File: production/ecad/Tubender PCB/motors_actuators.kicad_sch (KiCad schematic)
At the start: 5 parts, among them J2 1729157, J3 1729157, J4 1729157, J5 1729157, J6 1729186

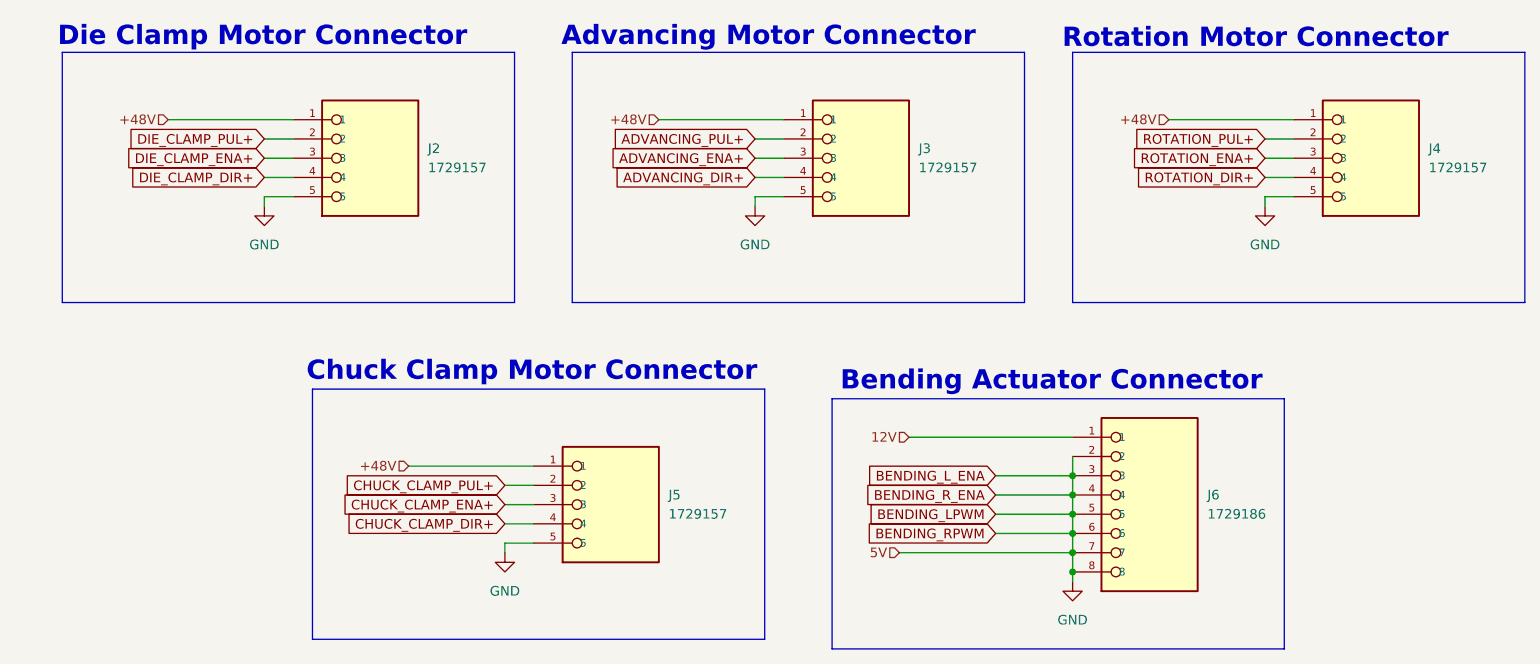
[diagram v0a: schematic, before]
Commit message: final for rev 1
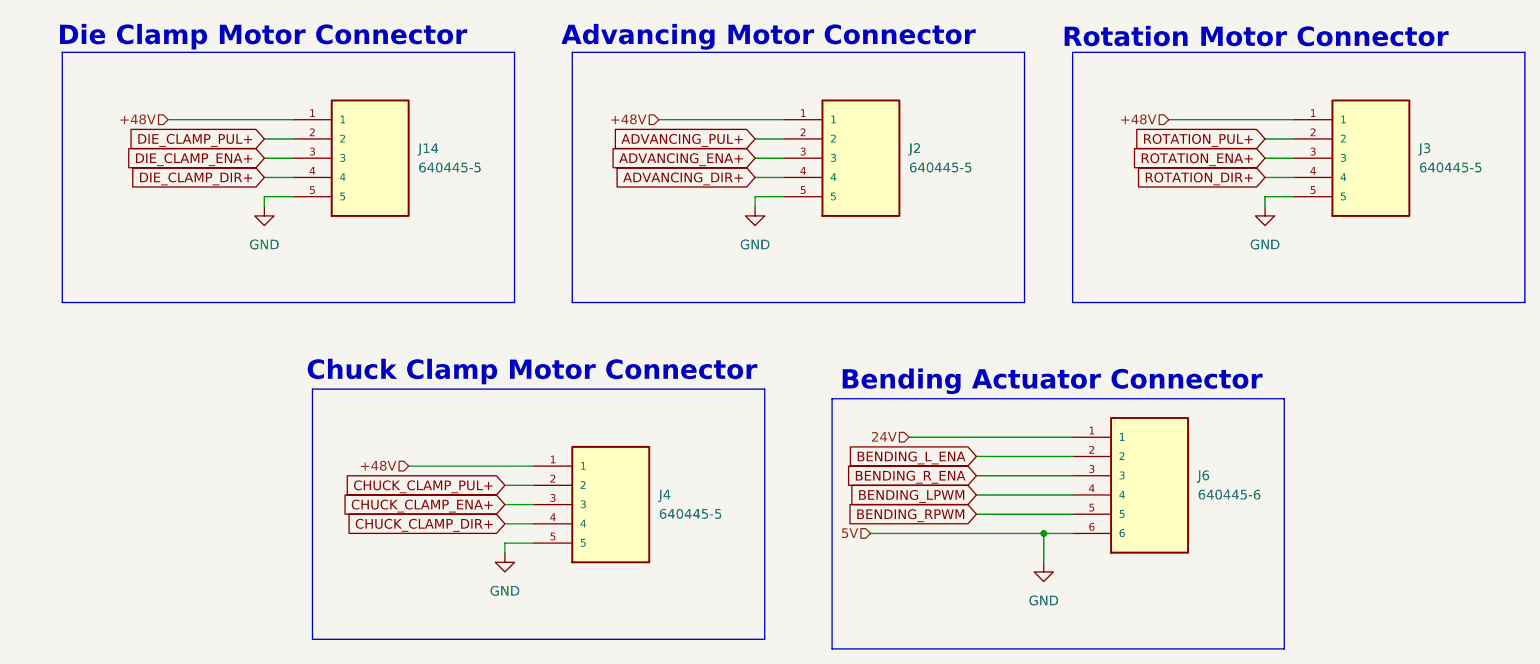
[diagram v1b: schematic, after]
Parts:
- removed J2, J3, J4, J5: 1729157, 1729157:PHOENIX_1729157, symbol 1729157:1729157
- removed J6: 1729186, 1729186:PHOENIX_1729186, symbol 1729186:1729186
- added J14, J2, J3, J4: 640445-5, 640445-5:TE_640445-5, symbol 640445-5:640445-5
- added J6: 640445-6, 640445-6:TE_640445-6, symbol 640445-6:640445-6
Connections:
- net +48V: now also J14.1, J2.1, J3.1, J4.1
- net ADVANCING_DIR+: now also J2.4
- net ADVANCING_ENA+: now also J2.3
- net ADVANCING_PUL+: now also J2.2
- net CHUCK_CLAMP_DIR+: now also J4.4
- net CHUCK_CLAMP_ENA+: now also J4.3
- net CHUCK_CLAMP_PUL+: now also J4.2
- net DIE_CLAMP_DIR+: now also J14.4
- net DIE_CLAMP_ENA+: now also J14.3
- net DIE_CLAMP_PUL+: now also J14.2
- net GND: now also J14.5, J2.5, J3.5, J4.5, J6.6
- net ROTATION_DIR+: now also J3.4
- net ROTATION_ENA+: now also J3.3
- net ROTATION_PUL+: now also J3.2
- new net 24V: J6.1
- new net BENDING_LPWM: J6.4
- new net BENDING_L_ENA: J6.2
- new net BENDING_RPWM: J6.5
- new net BENDING_R_ENA: J6.3
